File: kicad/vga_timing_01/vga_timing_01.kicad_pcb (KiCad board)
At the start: 2 copper layers, 45.7 x 45.7 mm, 10 parts, among them J1 Conn_02x01, U1 74LS393, U2 74LS393, U3 74LS393, U4 PAL20RS10, U5 PAL20RS10, X1 ACO-14MHz

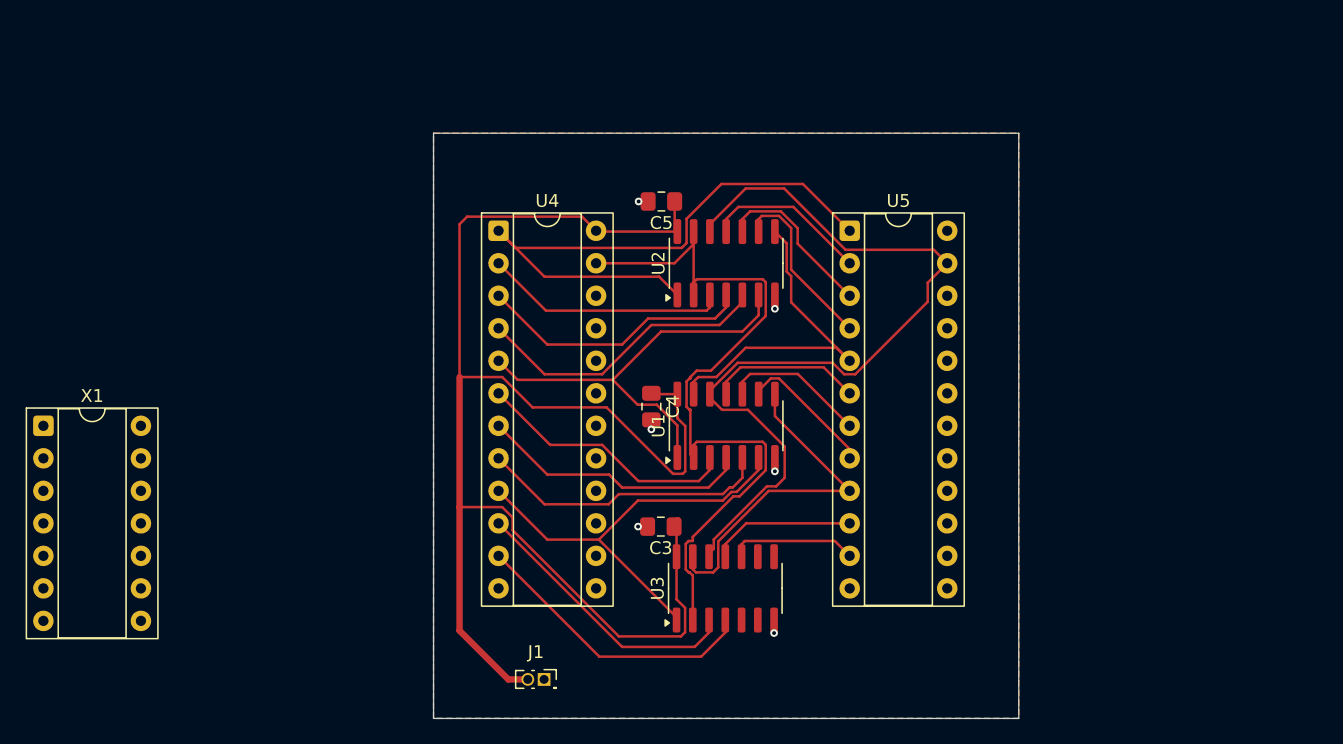
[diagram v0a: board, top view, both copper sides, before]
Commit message: vga timing board 01 work
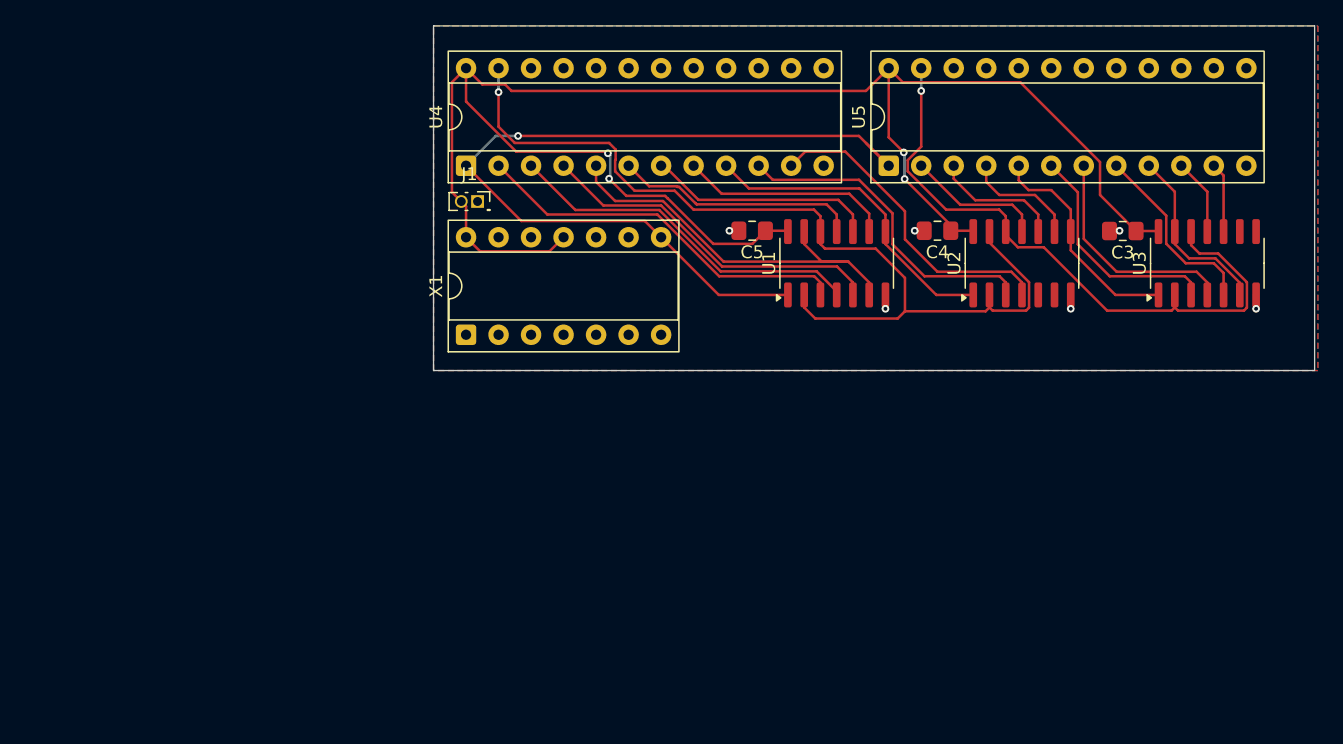
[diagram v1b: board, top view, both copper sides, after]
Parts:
- moved U3 45.4 mm to (121.4, 53.3)
- moved C3 42.8 mm to (114.8, 50.8)
- moved J1 37.7 mm to (64.4, 48.5)
- moved X1 33.8 mm to (63.5, 58.9), turned to 90 degrees
- moved C4 26.2 mm to (100.3, 50.8), turned to 180 degrees
- moved U2 23.1 mm to (106.9, 53.3)
- moved U1 15.4 mm to (92.5, 53.3)
- moved C5 7.45 mm to (85.9, 50.8)
- moved U5 5.92 mm to (96.5, 45.7), turned to 90 degrees
- moved U4 5.68 mm to (63.5, 45.7), turned to 90 degrees
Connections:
- U1 pad 1: /H03 -> /CLOCK
- U1 pad 10: /V05 -> /H05
- U1 pad 11: /V04 -> /H04
- U1 pad 12: /~{V_RES} -> /~{H_RES}
- U1 pad 13: /V03 -> /H03
- U1 pad 3: /H04 -> /H00
- U1 pad 4: /H05 -> /H01
- U1 pad 5: /H06 -> /H02
- U1 pad 6: /H07 -> /H03
- U1 pad 8: /V07 -> /H07
- U1 pad 9: /V06 -> /H06
- U2 pad 1: /CLOCK -> /H07
- U2 pad 3: /H00 -> /H08
- U2 pad 4: /H01 -> /H09
- U2 pad 5: /H02 -> /H10
- U2 pad 6: /H03 -> /H11
- U3 pad 1: /H07 -> /V03
- U3 pad 2: /~{H_RES} -> /~{V_RES}
- U3 pad 3: /H08 -> /V04
- U3 pad 4: /H09 -> /V05
- U3 pad 5: /H10 -> /V06
- U3 pad 6: /H11 -> /V07
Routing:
- net /CLOCK: track 48.7 -> 66.8 mm, vias 0 -> 1
- net VCC: track 119.3 -> 135.5 mm, vias 0 -> 4
- net /~{V_RES}: track 66.4 -> 50.3 mm, vias 0 -> 1
- net /V07: track 27.1 -> 14.2 mm
- net /~{H_RES}: track 62.0 -> 73.8 mm, vias 0 -> 1
- net /H00: track 19.1 -> 29.9 mm
- net /V03: track 27.2 -> 17.9 mm
- net /H07: track 33.9 -> 24.8 mm
- net /H01: track 21.5 -> 28.2 mm
- net /V05: track 11.3 -> 17.8 mm
- net /H06: track 23.0 -> 16.7 mm
- net /V04: track 11.9 -> 18.1 mm
- net /V08: track 11.4 -> 5.99 mm
- net /V02: track 13.7 -> 8.99 mm
- net /V09: track 10.0 -> 5.46 mm
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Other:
- board size 45.7 x 45.7 mm -> 68.8 x 26.9 mm
